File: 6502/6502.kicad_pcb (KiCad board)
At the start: 2 copper layers, 188.3 x 190.4 mm, 54 parts, among them J1 Conn_01x08, J10 Conn_02x20_Odd_Even, J11 Mini-DIN-6, J12 Conn_02x20_Odd_Even, J13 Jack-DC, J14 Conn_01x02, J2 Conn_01x08, J3 Conn_01x03, J4 Conn_02x20_Odd_Even, J5 Conn_01x08, J6 Conn_01x05, J7 Conn_02x20_Odd_Even, J8 Conn_01x02, J9 Conn_01x02, Q1 FQP47P06, SW1 SW_Push, SW2 SW_Push, U1 74LS08, U2 74LS154, U3 28C256, U4 ATF22V10C, U5 65C02S, U6 AS6C4008-55PCN, U7 6522, U8 6522, U9 NHD-0420H1Z, X1 ACO-4MHz

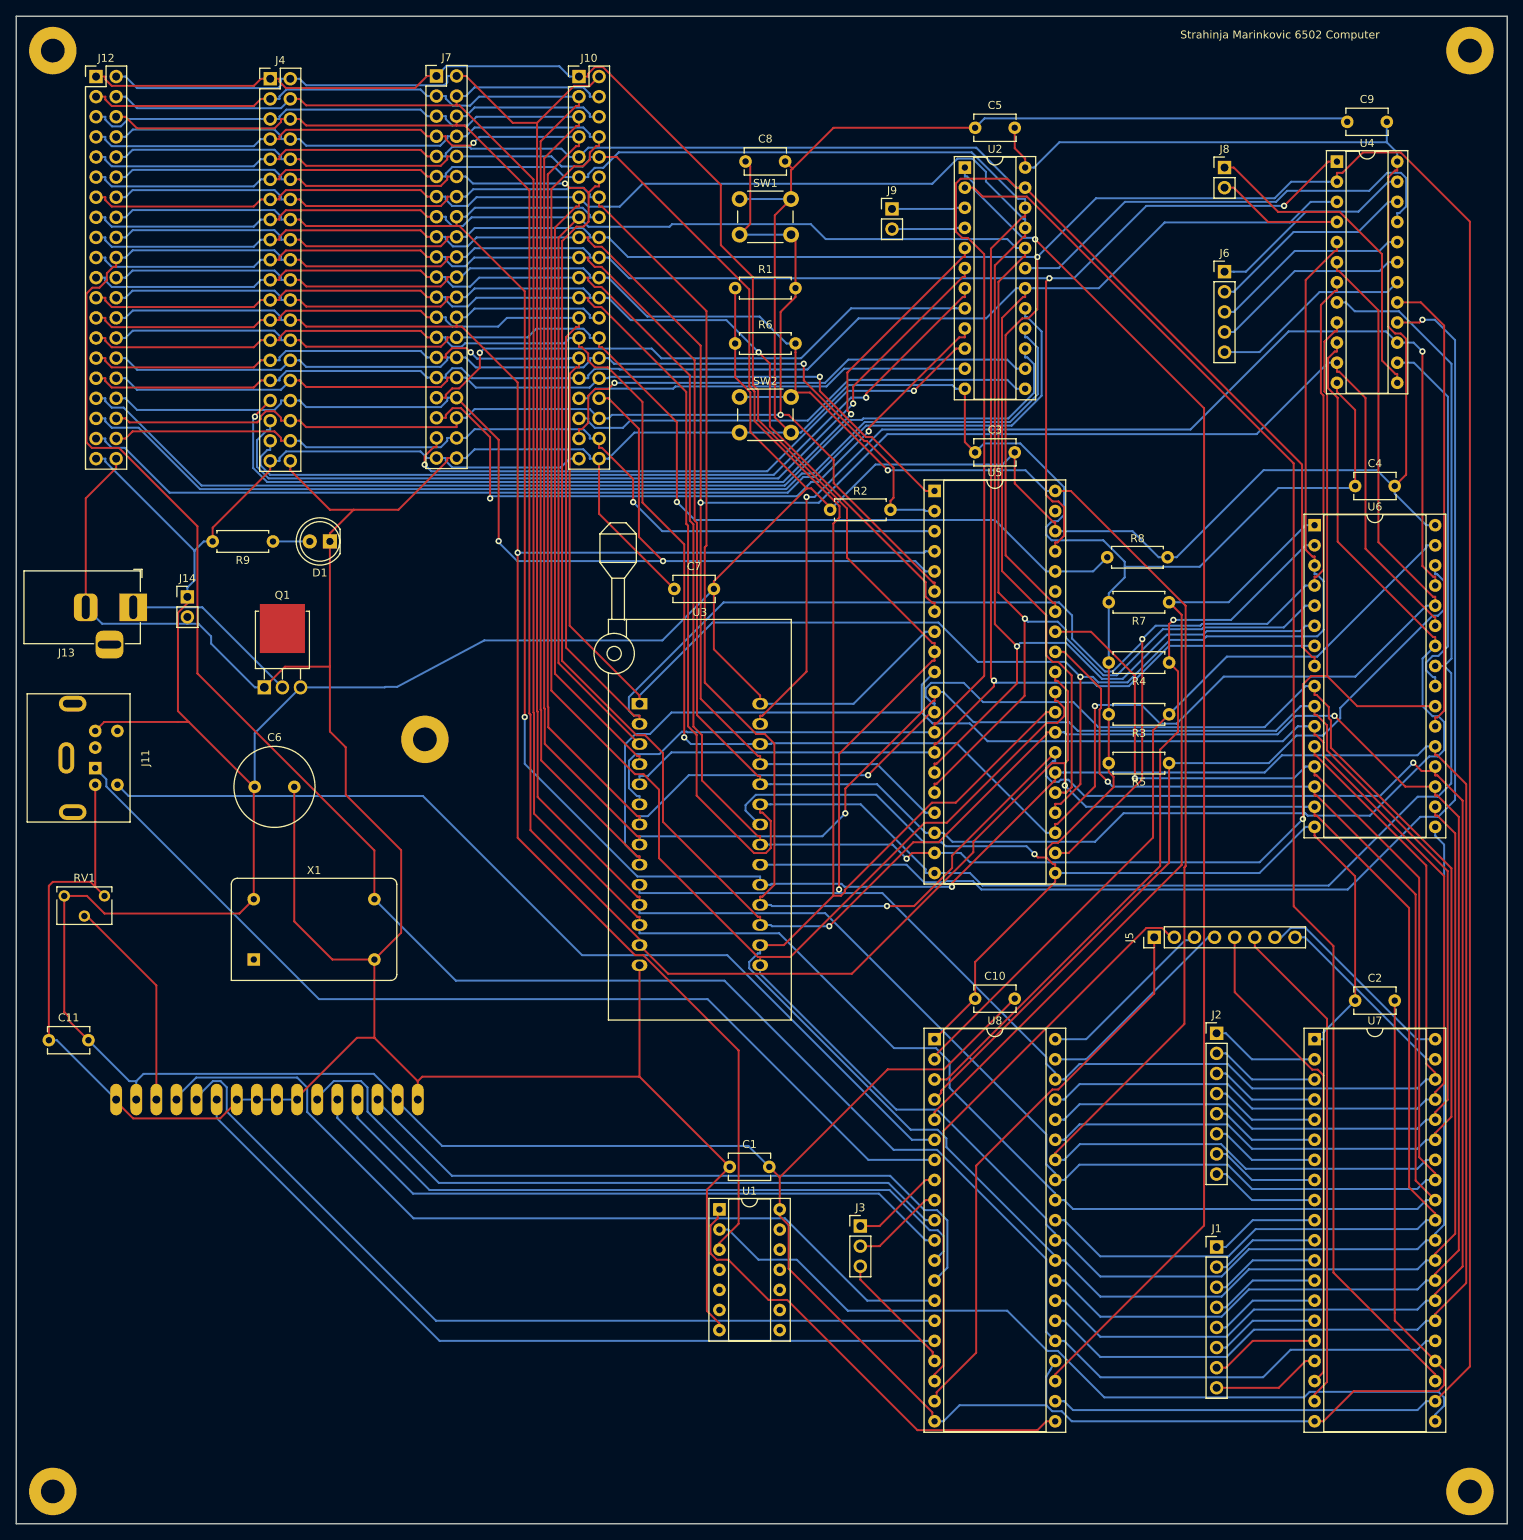
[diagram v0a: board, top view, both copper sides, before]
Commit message: updated pcb
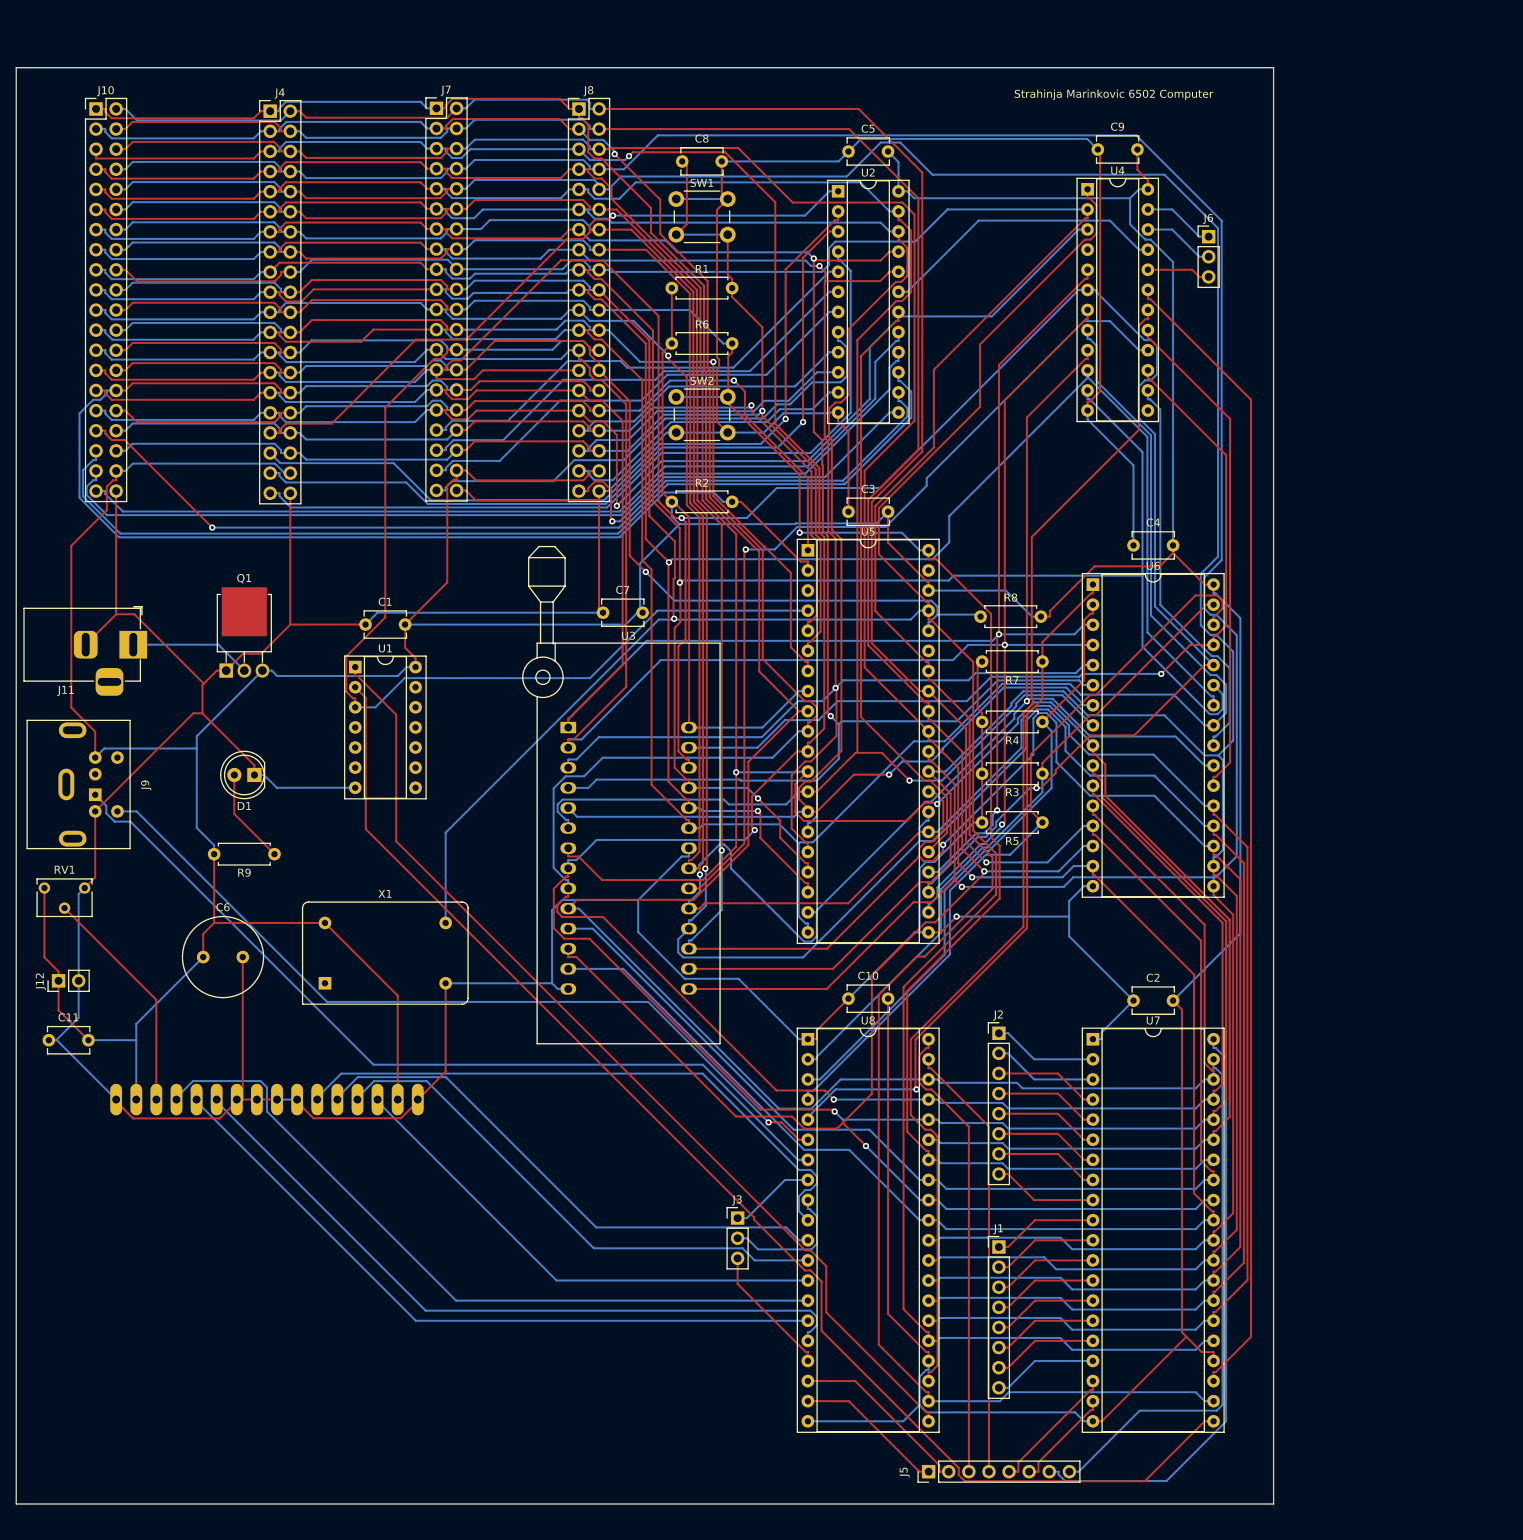
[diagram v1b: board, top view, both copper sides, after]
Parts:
- removed the J8 at (281.0, 91.8)
- removed the J9 at (239.0, 97.0)
- removed REF** (x5): MountingHole_3mm_Pad, MountingHole:MountingHole_3mm_Pad
- J6: value Conn_01x05 -> Conn_01x03; footprint Connector_PinHeader_2.54mm:PinHeader_1x05_P2.54mm_Vertical -> Connector_PinHeader_2.54mm:PinHeader_1x03_P2.54mm_Vertical
- moved C1 82.5 mm to (172.5, 149.5)
- moved U1 82.5 mm to (171.2, 154.9)
- moved J5 73.3 mm to (243.6, 256.5)
- moved J12 51.2 mm to (133.7, 194.5), turned to 90 degrees
- moved R9 39.5 mm to (161.0, 178.5)
- moved C9 31.7 mm to (265.0, 89.5)
- moved U4 31.7 mm to (263.7, 94.5)
- moved D1 31.0 mm to (158.5, 168.5)
- moved C4 29.0 mm to (269.5, 139.5)
- moved U6 29.0 mm to (264.4, 144.4)
- moved C2 28.0 mm to (269.5, 197.0)
- moved U7 28.0 mm to (264.4, 201.9)
- moved J1 27.5 mm to (252.5, 228.1)
- moved J2 27.5 mm to (252.5, 201.1)
- moved C6 22.5 mm to (152.0, 191.5)
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- renumbered J12 to J10, J13 to J11, J14 to J12, J10 to J8, J11 to J9
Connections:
- J10 pad 33: dev13 -> IO12
- J10 pad 35: dev14 -> IO13
- J10 pad 37: dev15 -> IO14
- J10 pad 38: PHI1O -> +5V
- J10 pad 39: +5V -> IO15
- J4 pad 33: dev4 -> IO0
- J4 pad 35: dev5 -> IO1
- J4 pad 37: dev6 -> IO2
- J4 pad 38: PHI1O -> +5V
- J4 pad 39: +5V -> IO3
- J7 pad 33: dev7 -> IO4
- J7 pad 35: dev8 -> IO5
- J7 pad 37: dev9 -> IO6
- J7 pad 38: PHI1O -> +5V
- J7 pad 39: +5V -> IO7
- J8 pad 33: dev10 -> IO8
- J8 pad 35: dev11 -> IO9
- J8 pad 37: dev12 -> IO10
- J8 pad 38: PHI1O -> +5V
- J8 pad 39: +5V -> IO11
- U2 pad 1: VIA1_CS -> IO0
- U2 pad 10: dev9 -> IO9
- U2 pad 11: dev10 -> IO10
- U2 pad 13: dev11 -> IO11
- U2 pad 14: dev12 -> IO12
- U2 pad 15: dev13 -> IO13
- U2 pad 16: dev14 -> IO14
- U2 pad 17: dev15 -> IO15
- U2 pad 2: VIA2_CS -> IO1
- U2 pad 3: dev2 -> IO2
- U2 pad 4: dev3 -> IO3
- U2 pad 5: dev4 -> IO4
- U2 pad 6: dev5 -> IO5
- U2 pad 7: dev6 -> IO6
- U2 pad 8: dev7 -> IO7
- U2 pad 9: dev8 -> IO8
- U4 pad 13: EXT_IN1 -> unconnected-(U4-Pad13)
- U4 pad 18: decode4 -> VIA1_CS
- U4 pad 19: decode3 -> VIA2_CS
- U4 pad 4: EXT_IN2 -> unconnected-(U4-Pad4)
- U5 pad 3: PHI1O -> unconnected-(U5-Pad3)
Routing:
- net GND: track 846.9 -> 682.8 mm
- net dev15: track 139.6 -> 0.00 mm
- net dev14: track 137.0 -> 0.00 mm
- net dev13: track 134.3 -> 0.00 mm
- net IO13: track 0.00 -> 125.8 mm
- net IO14: track 0.00 -> 118.1 mm
- net IO12: track 0.00 -> 117.2 mm, vias 0 -> 1
- net dev4: track 116.7 -> 0.00 mm, vias 2 -> 0
- net IO15: track 0.00 -> 115.4 mm
- net PHI1O: track 113.9 -> 0.00 mm, vias 1 -> 0
- net dev5: track 109.7 -> 0.00 mm, vias 1 -> 0
- net dev6: track 104.0 -> 0.00 mm, vias 1 -> 0
- net IO1: track 0.00 -> 101.1 mm, vias 0 -> 1
- net IO3: track 0.00 -> 100.4 mm
- net IO2: track 0.00 -> 100.0 mm, vias 0 -> 1
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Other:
- board size 188.3 x 190.4 mm -> 158.8 x 181.4 mm
